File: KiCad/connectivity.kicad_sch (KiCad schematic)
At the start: 15 parts, among them IC1 NRF7002-QFAA-R7, IC12 NRF54L15-QFAA-R, IC2 SARA-R410M-02B, U17 CXD5610GF, U19 HP5354.A, U21 BGA524N6, U23 BGA524N6, Y3 ECS-TXO-20CSMV4-260-AN-TR

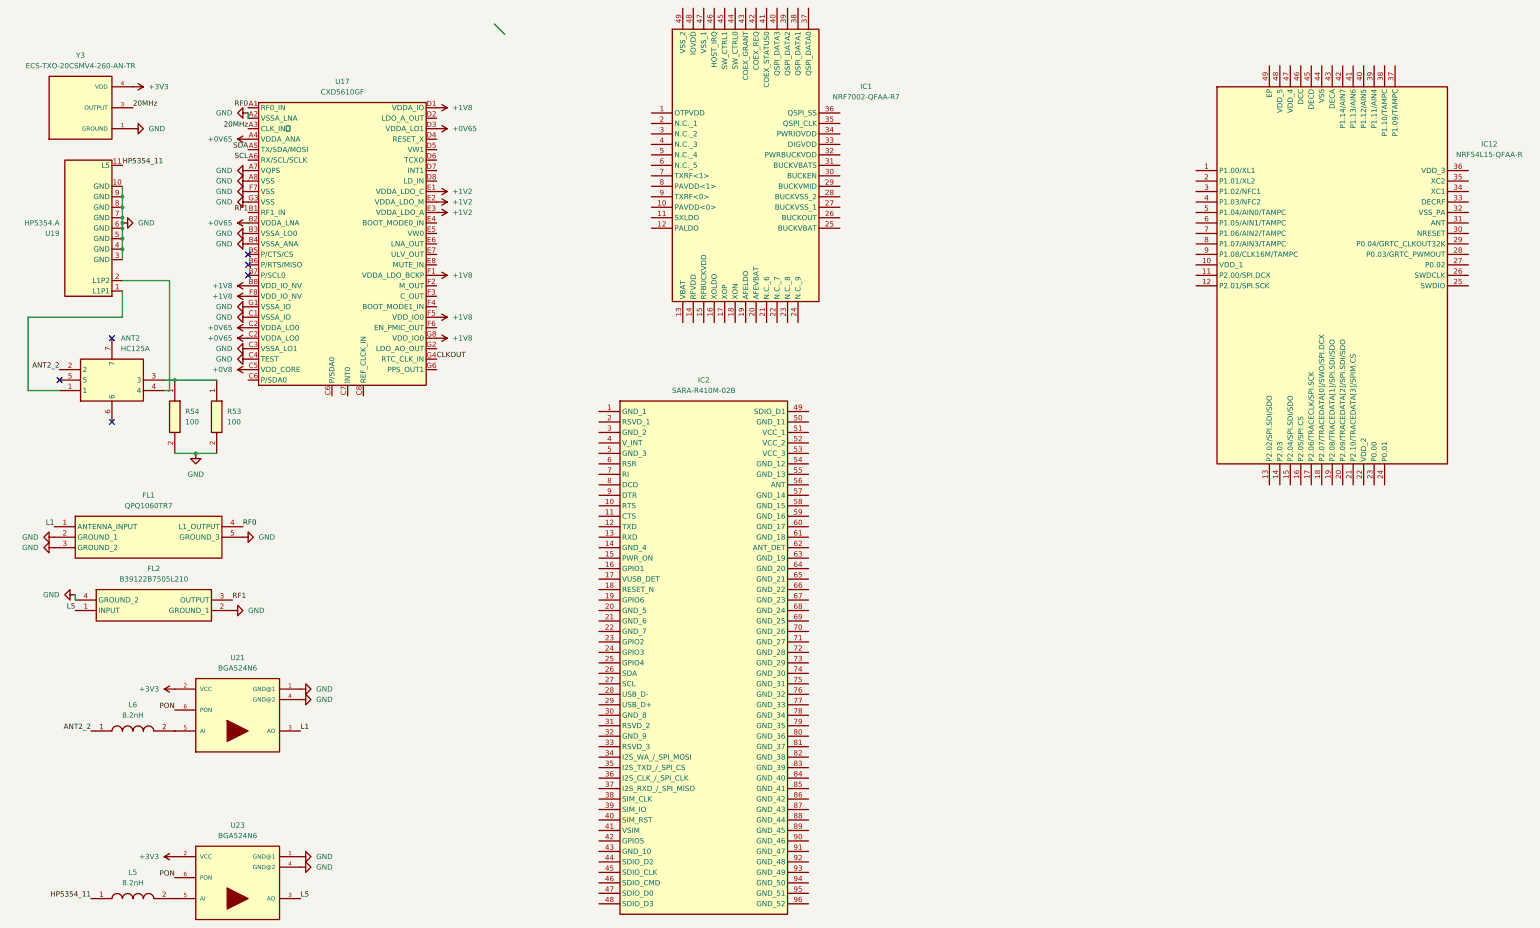
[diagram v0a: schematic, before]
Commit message: update
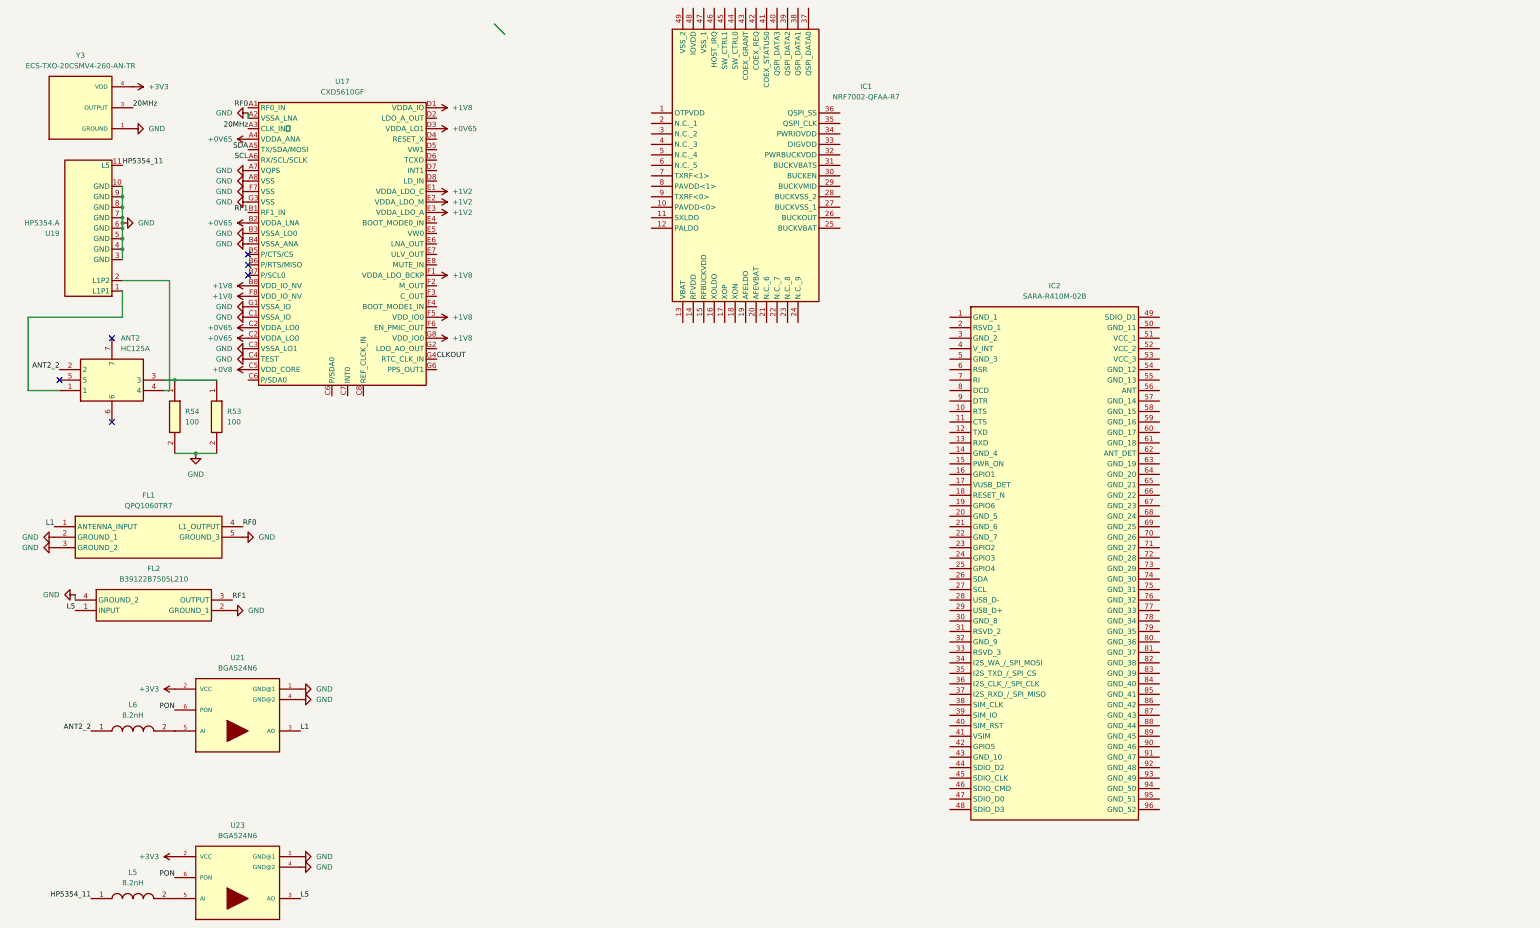
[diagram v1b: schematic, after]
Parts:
- removed IC12: NRF54L15-QFAA-R, QFN40P600X600X95-49N, symbol Symbols:NRF54L15-QFAA-R
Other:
- moved on the sheet: IC2
